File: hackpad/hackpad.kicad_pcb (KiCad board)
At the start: 2 copper layers, 48 x 66 mm, 7 parts, among them SW1 SW_Push, SW2 SW_Push, SW3 SW_Push, SW4 SW_Push, U1 XIAO-RP2040-DIP

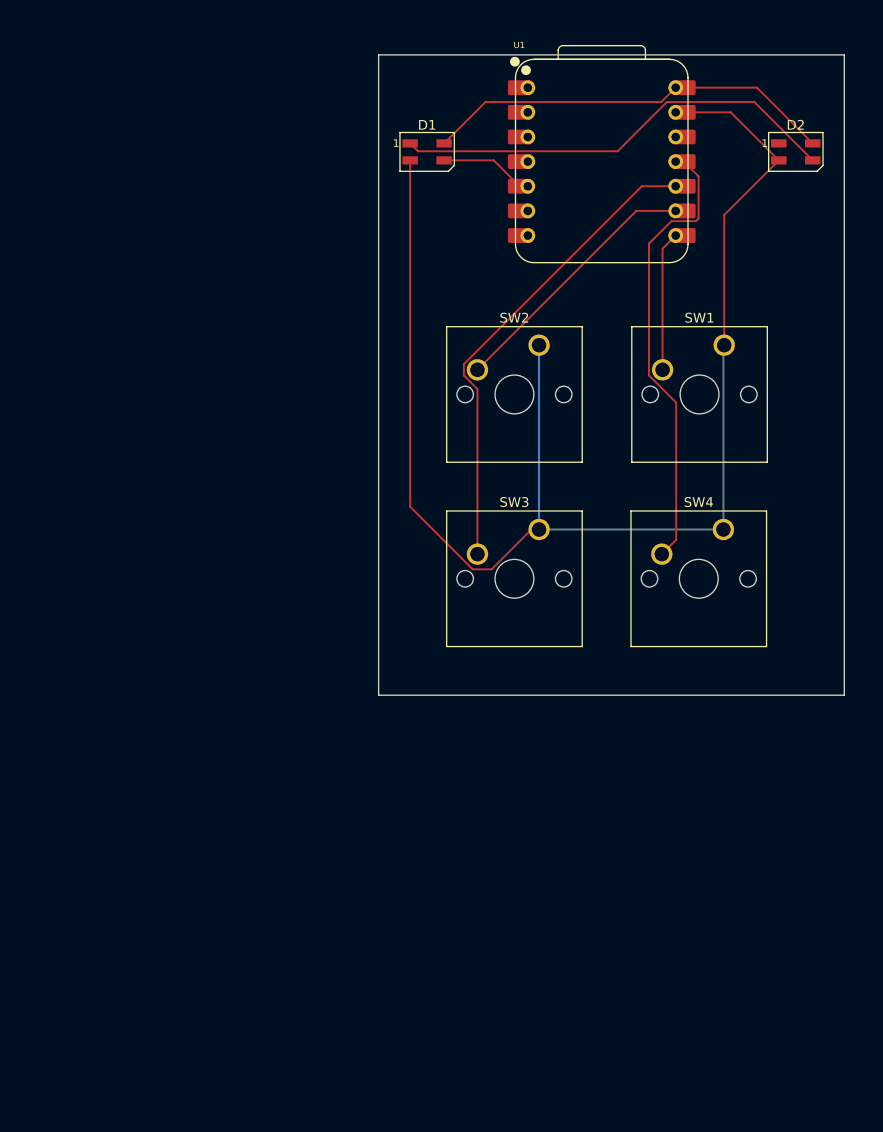
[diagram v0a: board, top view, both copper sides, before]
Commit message: v2 done?
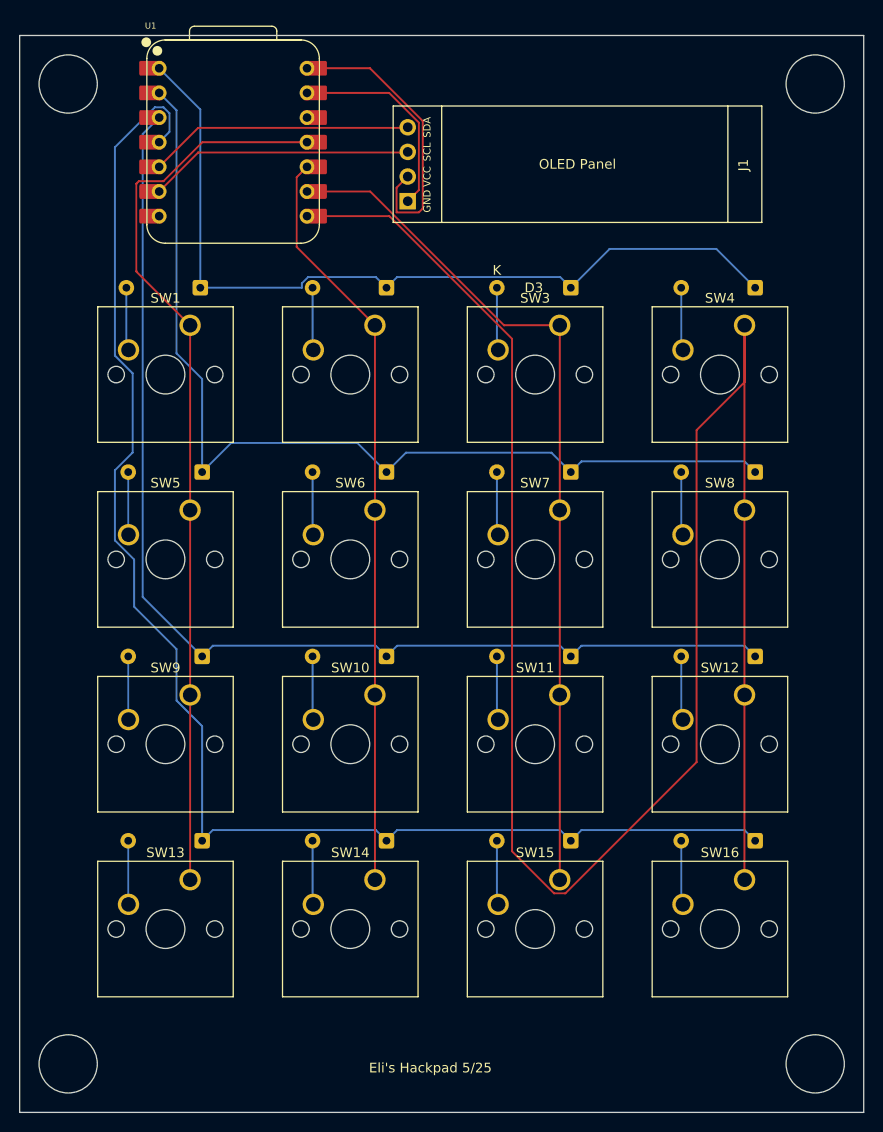
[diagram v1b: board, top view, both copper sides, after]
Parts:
- added D10: D, Diode_THT:D_DO-35_SOD27_P7.62mm_Horizontal, B.Cu at (157.8, 112.0)
- added D11: D, Diode_THT:D_DO-35_SOD27_P7.62mm_Horizontal, B.Cu at (176.8, 112.0)
- added D12: D, Diode_THT:D_DO-35_SOD27_P7.62mm_Horizontal, B.Cu at (195.8, 112.0)
- added D13: D, Diode_THT:D_DO-35_SOD27_P7.62mm_Horizontal, B.Cu at (138.8, 131.0)
- added D14: D, Diode_THT:D_DO-35_SOD27_P7.62mm_Horizontal, B.Cu at (157.8, 131.0)
- added D15: D, Diode_THT:D_DO-35_SOD27_P7.62mm_Horizontal, B.Cu at (176.8, 131.0)
- added D16: D, Diode_THT:D_DO-35_SOD27_P7.62mm_Horizontal, B.Cu at (195.8, 131.0)
- added D3: D, Diode_THT:D_DO-35_SOD27_P7.62mm_Horizontal, B.Cu at (176.8, 74.0)
- added D4: D, Diode_THT:D_DO-35_SOD27_P7.62mm_Horizontal, B.Cu at (195.8, 74.0)
- added D5: D, Diode_THT:D_DO-35_SOD27_P7.62mm_Horizontal, B.Cu at (138.8, 93.0)
- added D6: D, Diode_THT:D_DO-35_SOD27_P7.62mm_Horizontal, B.Cu at (157.8, 93.0)
- added D7: D, Diode_THT:D_DO-35_SOD27_P7.62mm_Horizontal, B.Cu at (176.8, 93.0)
- added D8: D, Diode_THT:D_DO-35_SOD27_P7.62mm_Horizontal, B.Cu at (195.8, 93.0)
- added D9: D, Diode_THT:D_DO-35_SOD27_P7.62mm_Horizontal, B.Cu at (138.8, 112.0)
- added J1: Conn_01x04_Pin, OLED:SSD1306-0.91-OLED-4pin-128x32, F.Cu at (196.5, 67.3)
- added SW10: SW_Push, Button_Switch_Keyboard:SW_Cherry_MX_1.00u_PCB, F.Cu at (156.6, 116.0)
- added SW11: SW_Push, Button_Switch_Keyboard:SW_Cherry_MX_1.00u_PCB, F.Cu at (175.7, 116.0)
- added SW12: SW_Push, Button_Switch_Keyboard:SW_Cherry_MX_1.00u_PCB, F.Cu at (194.7, 116.0)
- added SW13: SW_Push, Button_Switch_Keyboard:SW_Cherry_MX_1.00u_PCB, F.Cu at (137.6, 135.0)
- added SW14: SW_Push, Button_Switch_Keyboard:SW_Cherry_MX_1.00u_PCB, F.Cu at (156.6, 135.0)
- added SW15: SW_Push, Button_Switch_Keyboard:SW_Cherry_MX_1.00u_PCB, F.Cu at (175.7, 135.0)
- added SW16: SW_Push, Button_Switch_Keyboard:SW_Cherry_MX_1.00u_PCB, F.Cu at (194.7, 135.0)
- added SW5: SW_Push, Button_Switch_Keyboard:SW_Cherry_MX_1.00u_PCB, F.Cu at (137.6, 96.9)
- added SW6: SW_Push, Button_Switch_Keyboard:SW_Cherry_MX_1.00u_PCB, F.Cu at (156.6, 96.9)
- added SW7: SW_Push, Button_Switch_Keyboard:SW_Cherry_MX_1.00u_PCB, F.Cu at (175.7, 96.9)
- added SW8: SW_Push, Button_Switch_Keyboard:SW_Cherry_MX_1.00u_PCB, F.Cu at (194.7, 96.9)
- added SW9: SW_Push, Button_Switch_Keyboard:SW_Cherry_MX_1.00u_PCB, F.Cu at (137.6, 116.0)
- D1, D2: value SK6812MINI -> D; footprint LED_SMD:LED_SK6812MINI_PLCC4_3.5x3.5mm_P1.75mm -> Diode_THT:D_DO-35_SOD27_P7.62mm_Horizontal; moved to B.Cu
- moved SW1 55.1 mm to (137.6, 77.9)
- moved D2 44.5 mm to (157.8, 74.0), turned to 180 degrees
- moved U1 38.1 mm to (142.0, 59.0)
- moved D1 27.3 mm to (138.6, 74.0), turned to 180 degrees
- moved SW4 21.2 mm to (194.7, 77.9)
- moved SW3 21.2 mm to (175.7, 77.9)
- moved SW2 17.0 mm to (156.6, 77.9)
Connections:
- D1 pad 1: Net-(D1-DOUT) -> ROW0
- D1 pad 2: GND -> Net-(D1-A)
- D2 pad 1: unconnected-(D2-DOUT-Pad1) -> ROW0
- D2 pad 2: GND -> Net-(D2-A)
- SW1 pad 1: GND -> COL0
- SW1 pad 2: Net-(U1-GPIO1/RX) -> Net-(D1-A)
- SW2 pad 1: GND -> COL1
- SW2 pad 2: Net-(U1-GPIO2/SCK) -> Net-(D2-A)
- SW3 pad 1: GND -> COL2
- SW3 pad 2: Net-(U1-GPIO4/MISO) -> Net-(D3-A)
- SW4 pad 1: GND -> COL3
- SW4 pad 2: Net-(U1-GPIO3/MOSI) -> Net-(D4-A)
- U1 pad 1: unconnected-(U1-GPIO26/ADC0/A0-Pad1) -> ROW0
- U1 pad 10: Net-(U1-GPIO4/MISO) -> COL1
- U1 pad 11: Net-(U1-GPIO3/MOSI) -> COL0
- U1 pad 2: unconnected-(U1-GPIO27/ADC1/A1-Pad2) -> ROW1
- U1 pad 3: unconnected-(U1-GPIO28/ADC2/A2-Pad3) -> ROW2
- U1 pad 4: unconnected-(U1-GPIO29/ADC3/A3-Pad4) -> ROW3
- U1 pad 5: Net-(D1-DIN) -> SDA
- U1 pad 6: unconnected-(U1-GPIO7/SCL-Pad6) -> SCL
- U1 pad 8: Net-(U1-GPIO1/RX) -> COL3
- U1 pad 9: Net-(U1-GPIO2/SCK) -> COL2
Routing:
- net COL3: track 0.00 -> 209.9 mm
- net ROW3: track 0.00 -> 147.5 mm
- net GND: track 144.1 -> 21.4 mm
- net ROW2: track 0.00 -> 118.5 mm
- net ROW1: track 0.00 -> 103.0 mm
- net COL0: track 0.00 -> 93.4 mm
- net COL2: track 0.00 -> 88.9 mm
- net ROW0: track 0.00 -> 87.0 mm
- net COL1: track 0.00 -> 77.3 mm
- net Net-(U1-GPIO4/MISO): track 49.6 -> 0.00 mm
- net Net-(U1-GPIO3/MOSI): track 47.3 -> 0.00 mm
- net Net-(D1-DOUT): track 46.4 -> 0.00 mm
- net SDA: track 0.00 -> 27.3 mm
- net SCL: track 0.00 -> 27.3 mm
- net Net-(U1-GPIO2/SCK): track 27.2 -> 0.00 mm
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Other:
- board size 48 x 66 mm -> 87 x 111 mm
- board text added: "Eli's Hackpad 5/25"
